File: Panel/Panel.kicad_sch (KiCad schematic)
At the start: 68 parts, among them J1 Conn_01x03, J10 Conn_01x02, J11 Conn_01x02, J12 Conn_01x02, J2 USB_C_Receptacle_USB2.0, J3 Conn_01x02, J4 Conn_02x06_Odd_Even, J5 Conn_01x02, J6 Conn_01x02, J7 Conn_01x02, J8 Conn_01x02, J9 Conn_01x02, SW1 SW_Push, SW2 SW_Push, U1 W25Q32JVSS, U2 RP2040, U3 NCP1117-3.3_SOT223, Y1 12.000MHz

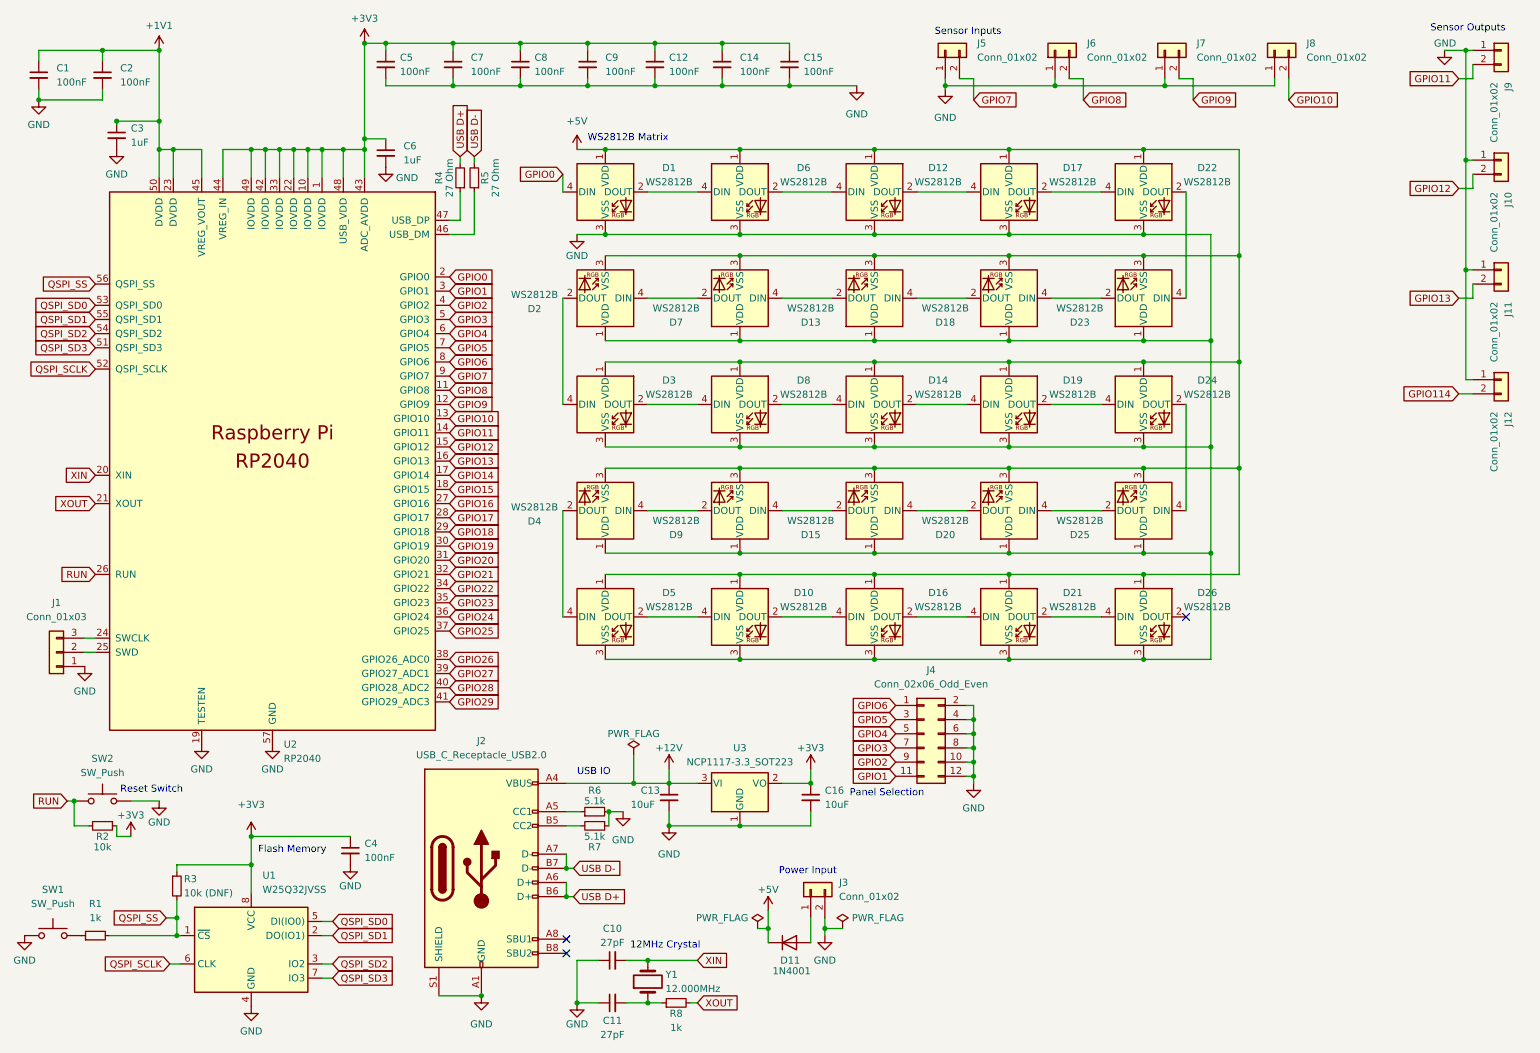
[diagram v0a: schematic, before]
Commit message: 90% routed
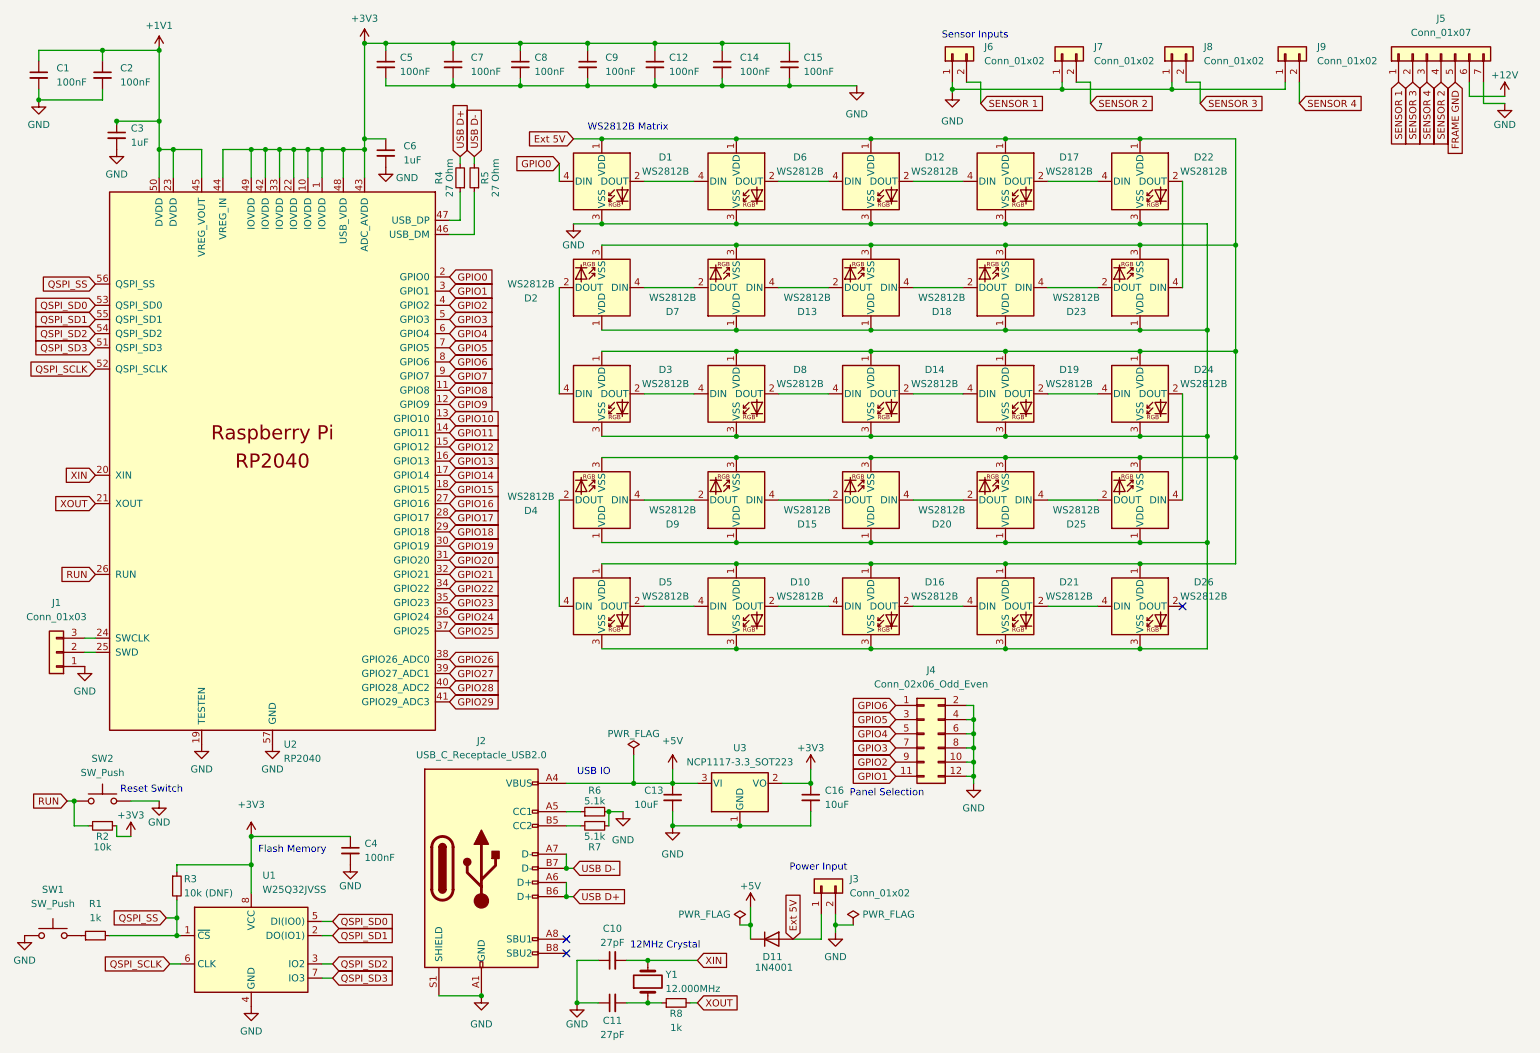
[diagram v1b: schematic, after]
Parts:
- removed J10, J11, J12, J5: Conn_01x02, Connector_Molex:Molex_Mini-Fit_Jr_5569-02A1_2x01_P4.20mm_Horizontal, symbol Connector_Generic:Conn_01x02
- added J5: Conn_01x07, 35312-XX60:35312-0760, symbol Connector_Generic:Conn_01x07
- J3: footprint Connector_JST:JST_XH_B2B-XH-AM_1x02_P2.50mm_Vertical -> Connector_JST:JST_XH_B2B-XH-A_1x02_P2.50mm_Vertical
- J6, J7, J8, J9: footprint Connector_Molex:Molex_Mini-Fit_Jr_5569-02A1_2x01_P4.20mm_Horizontal -> Connector_Molex:Molex_Mini-Fit_Jr_5569-02A2_2x01_P4.20mm_Horizontal
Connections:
- net +12V: now also J5.6 (Pin_6); no longer C13.1, J2.A4 (VBUS), J2.A9 (VBUS), J2.B4 (VBUS), J2.B9 (VBUS), U3.3 (VI)
- net +5V: now also C13.1, J2.A4 (VBUS), J2.A9 (VBUS), J2.B4 (VBUS), J2.B9 (VBUS), U3.3 (VI); no longer D1.1 (VDD), D10.1 (VDD), D12.1 (VDD), D13.3 (VSS), D14.1 (VDD), D15.3 (VSS), D16.1 (VDD), D17.1 (VDD), D18.3 (VSS), D19.1 (VDD), D2.3 (VSS), D20.3 (VSS), D21.1 (VDD), D22.1 (VDD), D23.3 (VSS), D24.1 (VDD), D25.3 (VSS), D26.1 (VDD), D3.1 (VDD), D4.3 (VSS), D5.1 (VDD), D6.1 (VDD), D7.3 (VSS), D8.1 (VDD), D9.3 (VSS)
- net GND: now also J5.7 (Pin_7)
- net GPIO10: no longer J8.2 (Pin_2)
- net GPIO11: no longer J9.2 (Pin_2)
- net GPIO8: no longer J6.2 (Pin_2)
- net GPIO9: no longer J7.2 (Pin_2)
- net Ext 5V: now reaches D11.2 (A), J3.1 (Pin_1)
- net Ext 5V: now also D1.1 (VDD), D10.1 (VDD), D12.1 (VDD), D13.3 (VSS), D14.1 (VDD), D15.3 (VSS), D16.1 (VDD), D17.1 (VDD), D18.3 (VSS), D19.1 (VDD), D2.3 (VSS), D20.3 (VSS), D21.1 (VDD), D22.1 (VDD), D23.3 (VSS), D24.1 (VDD), D25.3 (VSS), D26.1 (VDD), D3.1 (VDD), D4.3 (VSS), D5.1 (VDD), D6.1 (VDD), D7.3 (VSS), D8.1 (VDD), D9.3 (VSS)
- new net FRAME GND: J5.5 (Pin_5)
- new net SENSOR 1: J5.1 (Pin_1), J6.2 (Pin_2)
- new net SENSOR 2: J5.4 (Pin_4), J7.2 (Pin_2)
- new net SENSOR 3: J5.2 (Pin_2), J8.2 (Pin_2)
- new net SENSOR 4: J5.3 (Pin_3), J9.2 (Pin_2)
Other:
- note removed: "Sensor Outputs"
- moved on the sheet: C13, D1, D10, D11, D12, D13, D14, D15, D16, D17, D18, D19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
